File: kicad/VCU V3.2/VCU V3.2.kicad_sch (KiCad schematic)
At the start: 12 parts, among them J1 AVR-ISP-6, SW1 SW_Push, U1 ATmega328P-A, Y1 16MHz

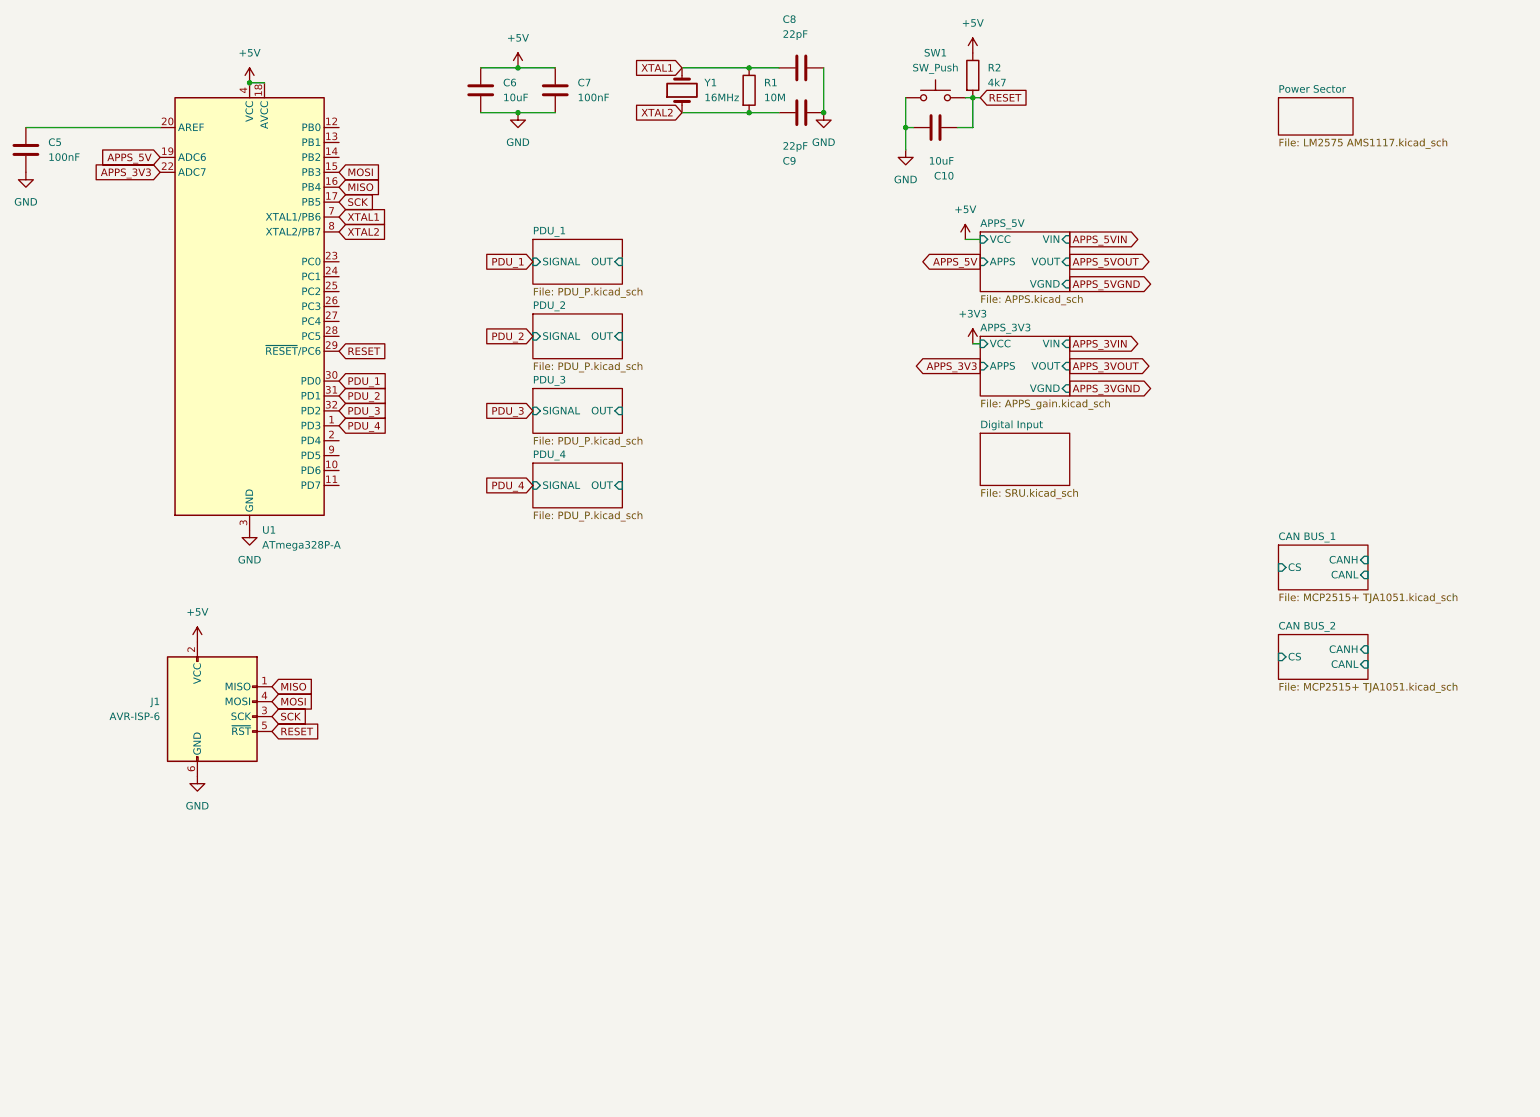
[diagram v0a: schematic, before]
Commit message: VCU V3.2
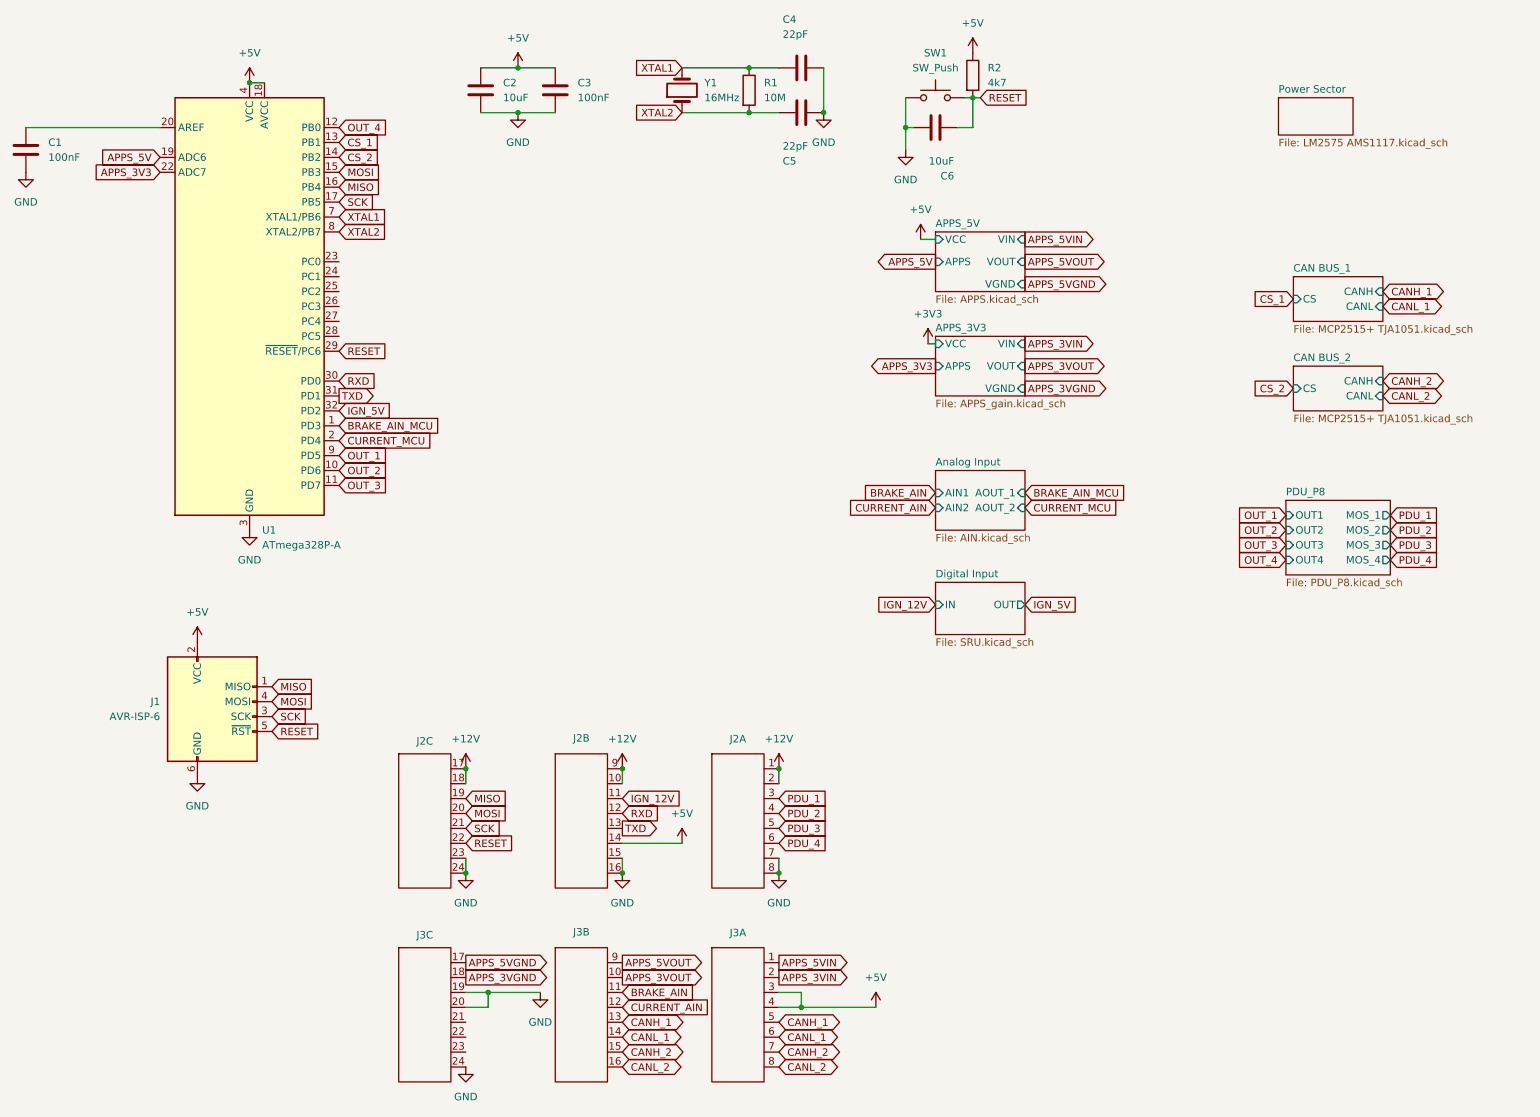
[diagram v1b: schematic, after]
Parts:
- added J2: ~, Better_Handsolder:HD241_24pin, symbol HD241:HD241
- added J3: ~, Better_Handsolder:HD241_GF30, symbol HD241:HD241
- renumbered C5 to C1, C6 to C2, C7 to C3, C8 to C4, C9 to C5, C10 to C6
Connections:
- net +5V: now also J2.14, J3.3, J3.4
- net APPS_3VGND: now also J3.18
- net APPS_3VIN: now also J3.2
- net APPS_3VOUT: now also J3.10
- net APPS_5VGND: now also J3.17
- net APPS_5VIN: now also J3.1
- net APPS_5VOUT: now also J3.9
- net GND: now also J2.15, J2.16, J2.23, J2.24, J2.7, J2.8, J3.19, J3.20, J3.24
- net MISO: now also J2.19
- net MOSI: now also J2.20
- net PDU_1: now also J2.3; no longer U1.30 (PD0)
- net PDU_2: now also J2.4; no longer U1.31 (PD1)
- net PDU_3: now also J2.5; no longer U1.32 (PD2)
- net PDU_4: now also J2.6; no longer U1.1 (PD3)
- net RESET: now also J2.22
- net SCK: now also J2.21
- net OUT_2: now reaches U1.10 (PD6)
- net OUT_3: now reaches U1.11 (PD7)
- net OUT_4: now reaches U1.12 (PB0)
- net CS_1: now reaches U1.13 (PB1)
- net CS_2: now reaches U1.14 (PB2)
- net CURRENT_MCU: now reaches U1.2 (PD4)
- net OUT_1: now reaches U1.9 (PD5)
- new net +12V: J2.1, J2.10, J2.17, J2.18, J2.2, J2.9
- new net BRAKE_AIN: J3.11
- new net BRAKE_AIN_MCU: U1.1 (PD3)
- new net CANH_1: J3.13, J3.5
- new net CANH_2: J3.15, J3.7
- new net CANL_1: J3.14, J3.6
- new net CANL_2: J3.16, J3.8
- new net CURRENT_AIN: J3.12
- new net IGN_12V: J2.11
- new net IGN_5V: U1.32 (PD2)
- new net RXD: J2.12, U1.30 (PD0)
- new net TXD: J2.13, U1.31 (PD1)
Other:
- removed sheet PDU_1
- removed sheet PDU_2
- removed sheet PDU_3
- removed sheet PDU_4
- added sheet Analog Input (AIN.kicad_sch)
- added sheet PDU_P8 (PDU_P8.kicad_sch)
- sheet Digital Input ports: added IN, OUT; removed none
